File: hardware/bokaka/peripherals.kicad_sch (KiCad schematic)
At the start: 50 parts, among them U1 IS31FL3236A-QFLS2-TR

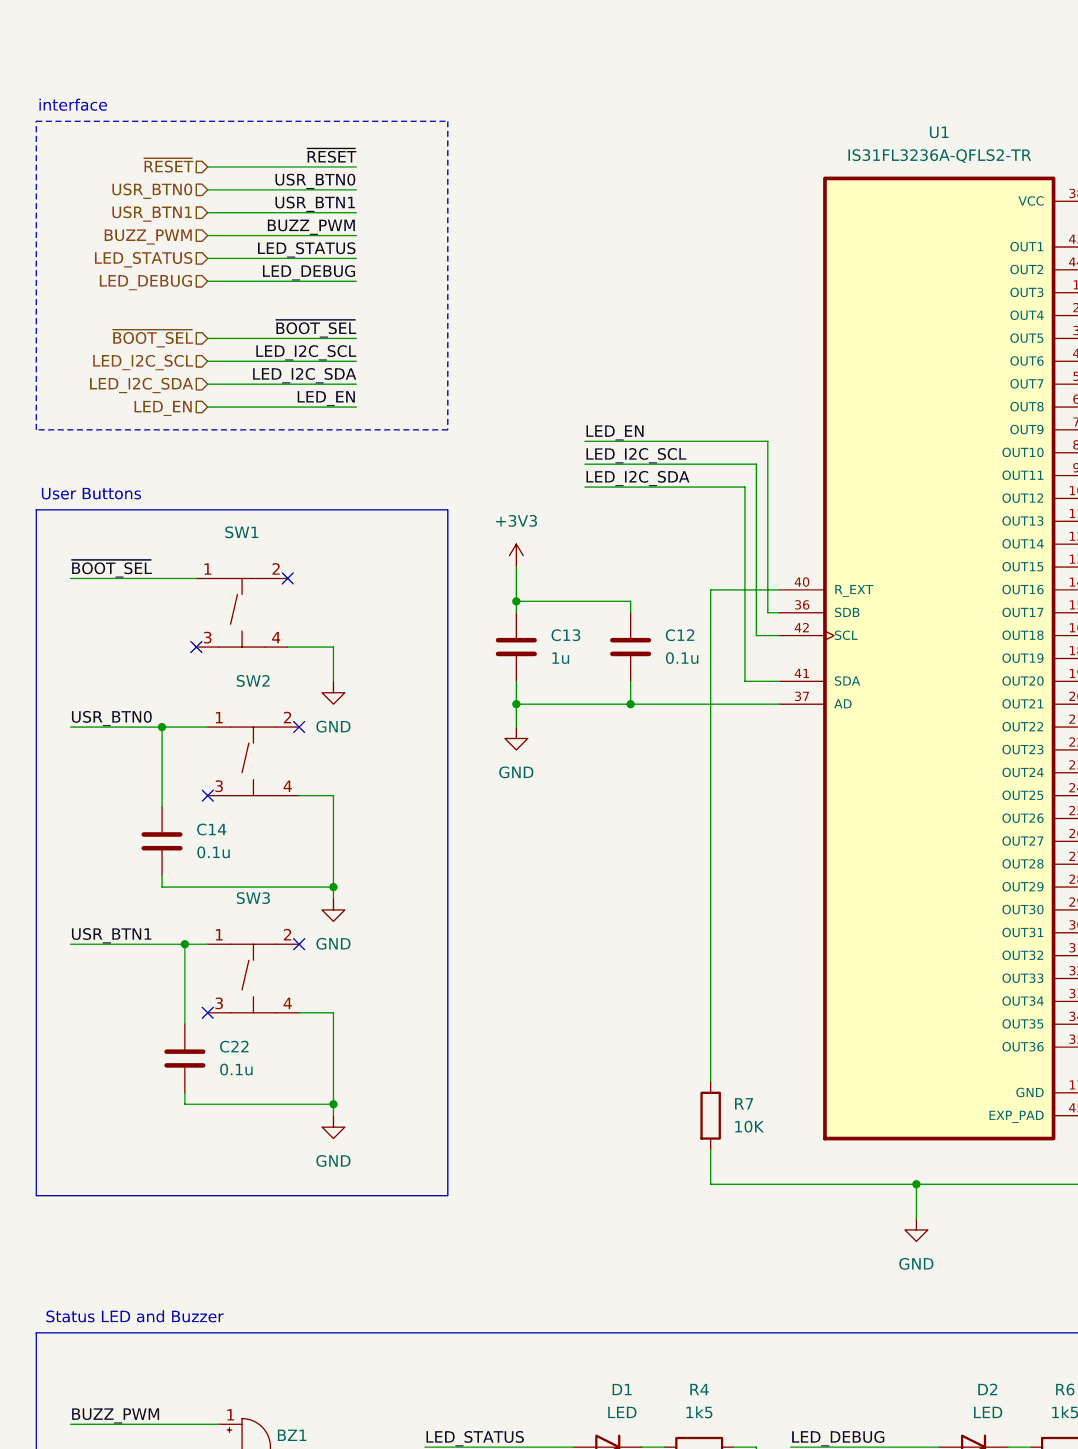
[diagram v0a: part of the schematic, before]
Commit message: hardware update
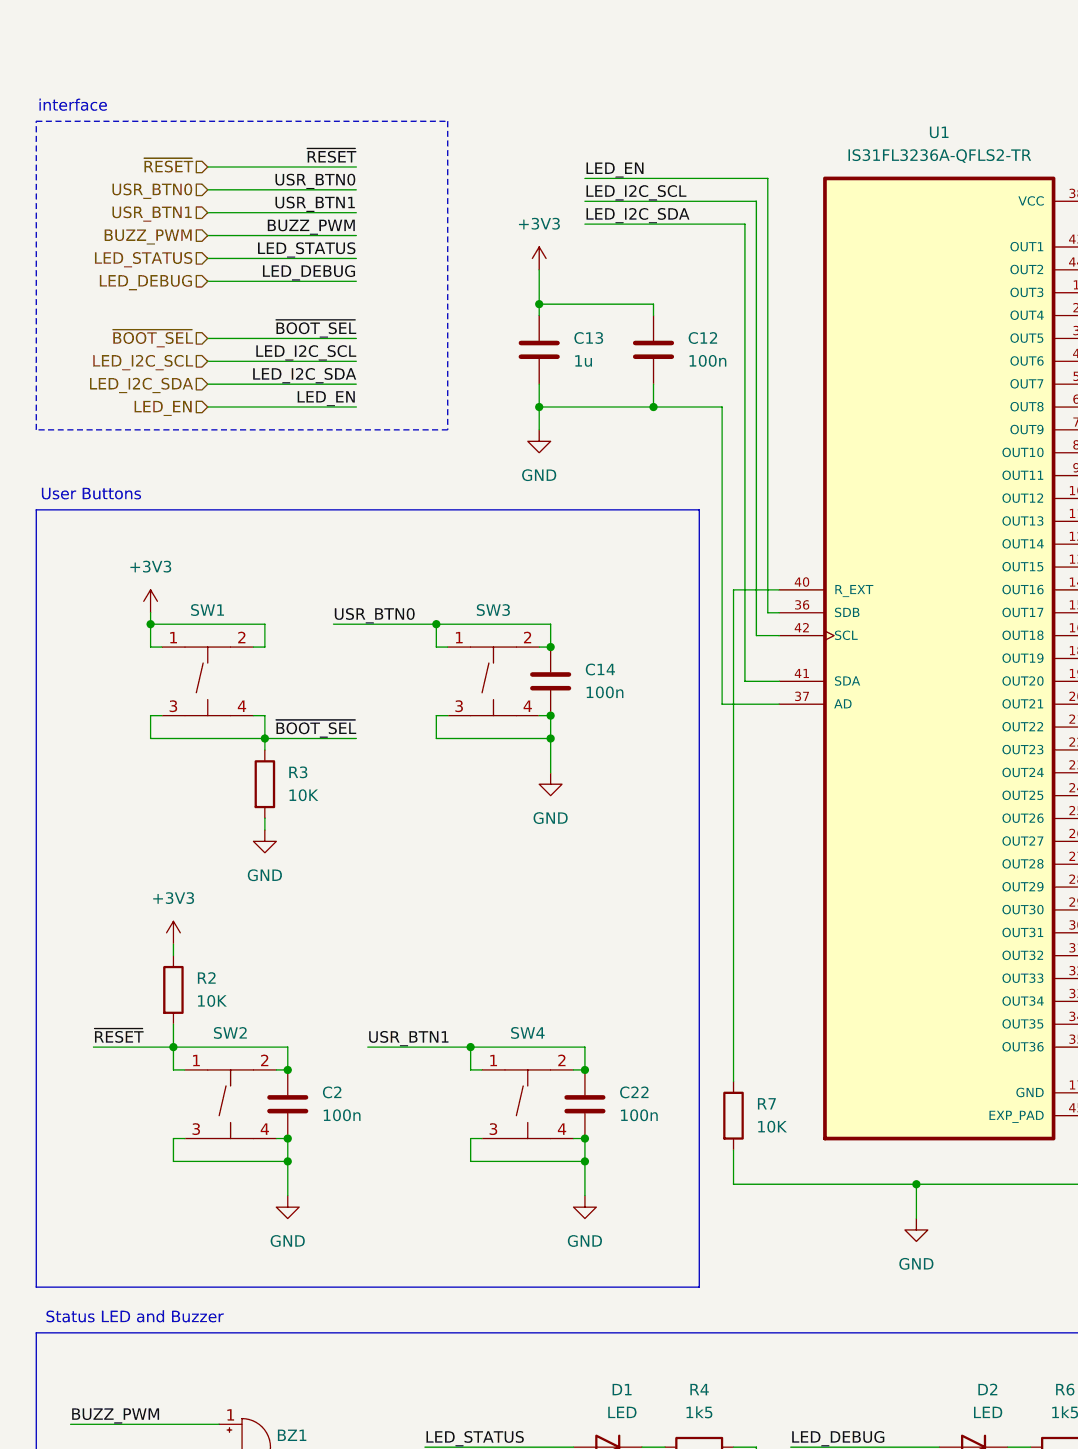
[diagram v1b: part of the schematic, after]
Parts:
- added C2: 100n, Capacitor_SMD:C_0402_1005Metric, symbol Device:C
- added R2, R3: 10K, Resistor_SMD:R_0402_1005Metric, symbol Device:R
- added SW4: ~, EasyEDA_Lib:SW-SMD_4P-L5.1-W5.1-P3.70-LS6.5-TL_H1.5, symbol Symbols:TS-1187A-B-A-B
- C12, C14, C22: value 0.1u -> 100n
- C13: footprint Capacitor_SMD:C_0402_1005Metric -> Capacitor_SMD:C_0603_1608Metric
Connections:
- net +3V3: now also SW1.1 (A), SW1.2 (B), R2.1
- net GND: now also SW2.3 (C), SW3.3 (C), C2.2, R3.2, SW4.3 (C), SW4.4 (D); no longer SW1.4 (D)
- net USR_BTN0: now also SW3.1 (A), SW3.2 (B); no longer SW2.1 (A)
- net USR_BTN1: now also SW4.1 (A), SW4.2 (B); no longer SW3.1 (A)
- net ~{BOOT_SEL}: now also SW1.3 (C), SW1.4 (D), R3.1; no longer SW1.1 (A)
- net ~{RESET}: now also SW2.1 (A), SW2.2 (B), C2.1, R2.2
- no-connect marks 6 -> 0
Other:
- moved on the sheet: C12, C13, R7, SW1

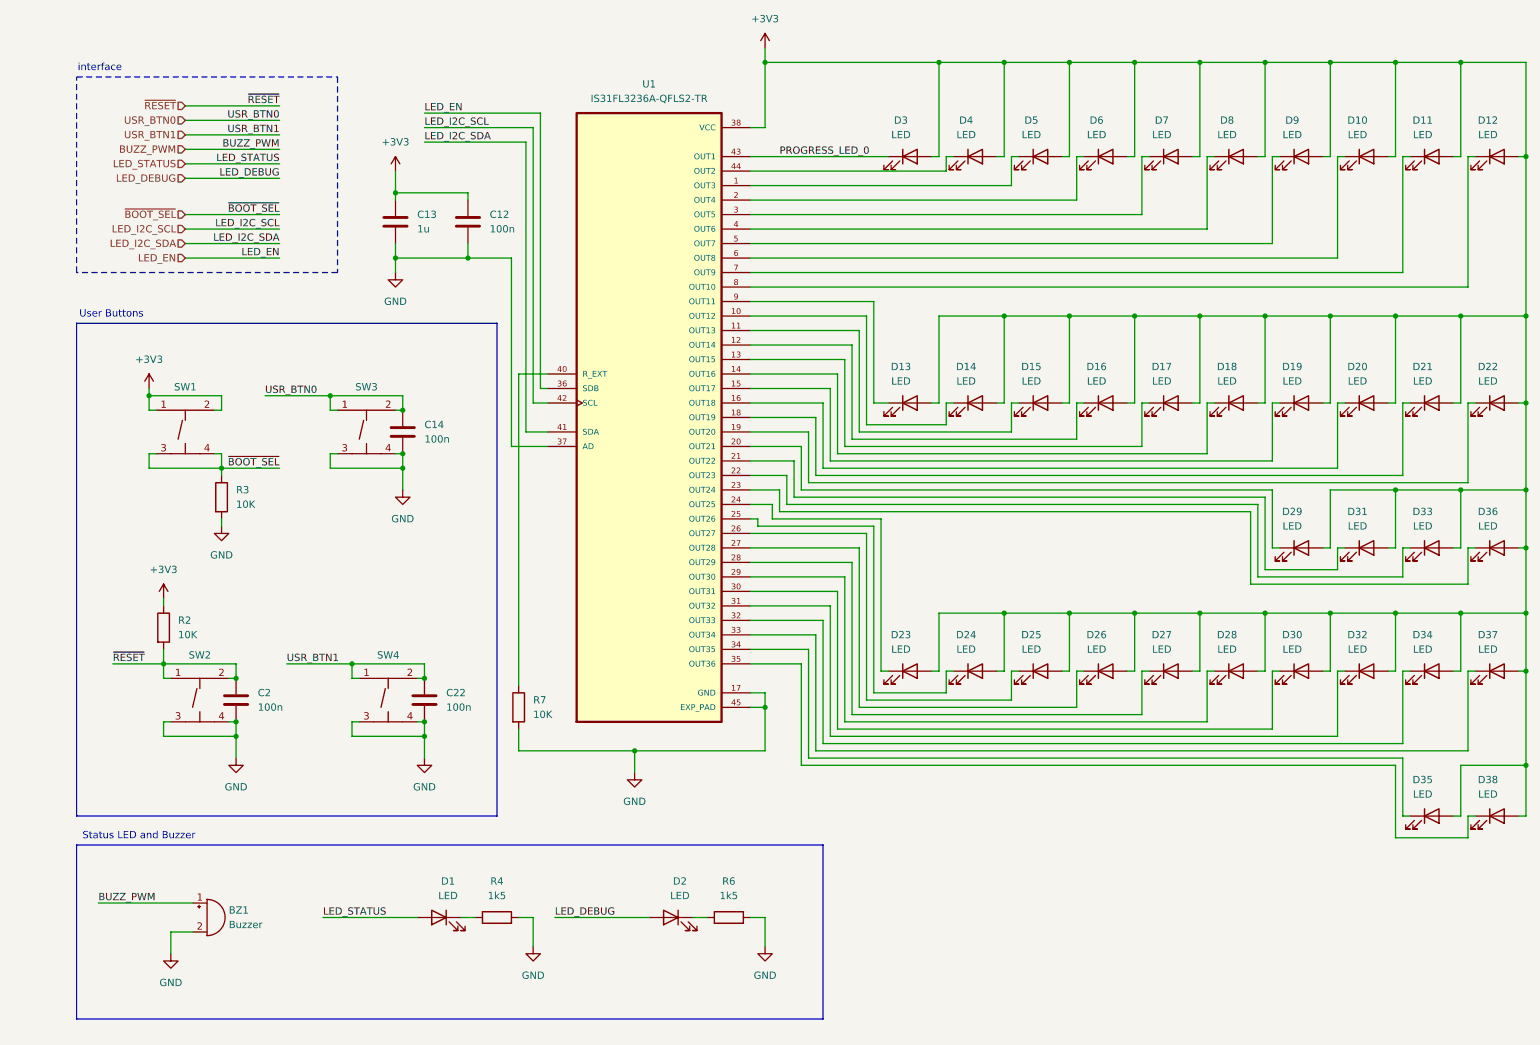
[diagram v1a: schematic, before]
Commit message: Devkit Production Ready
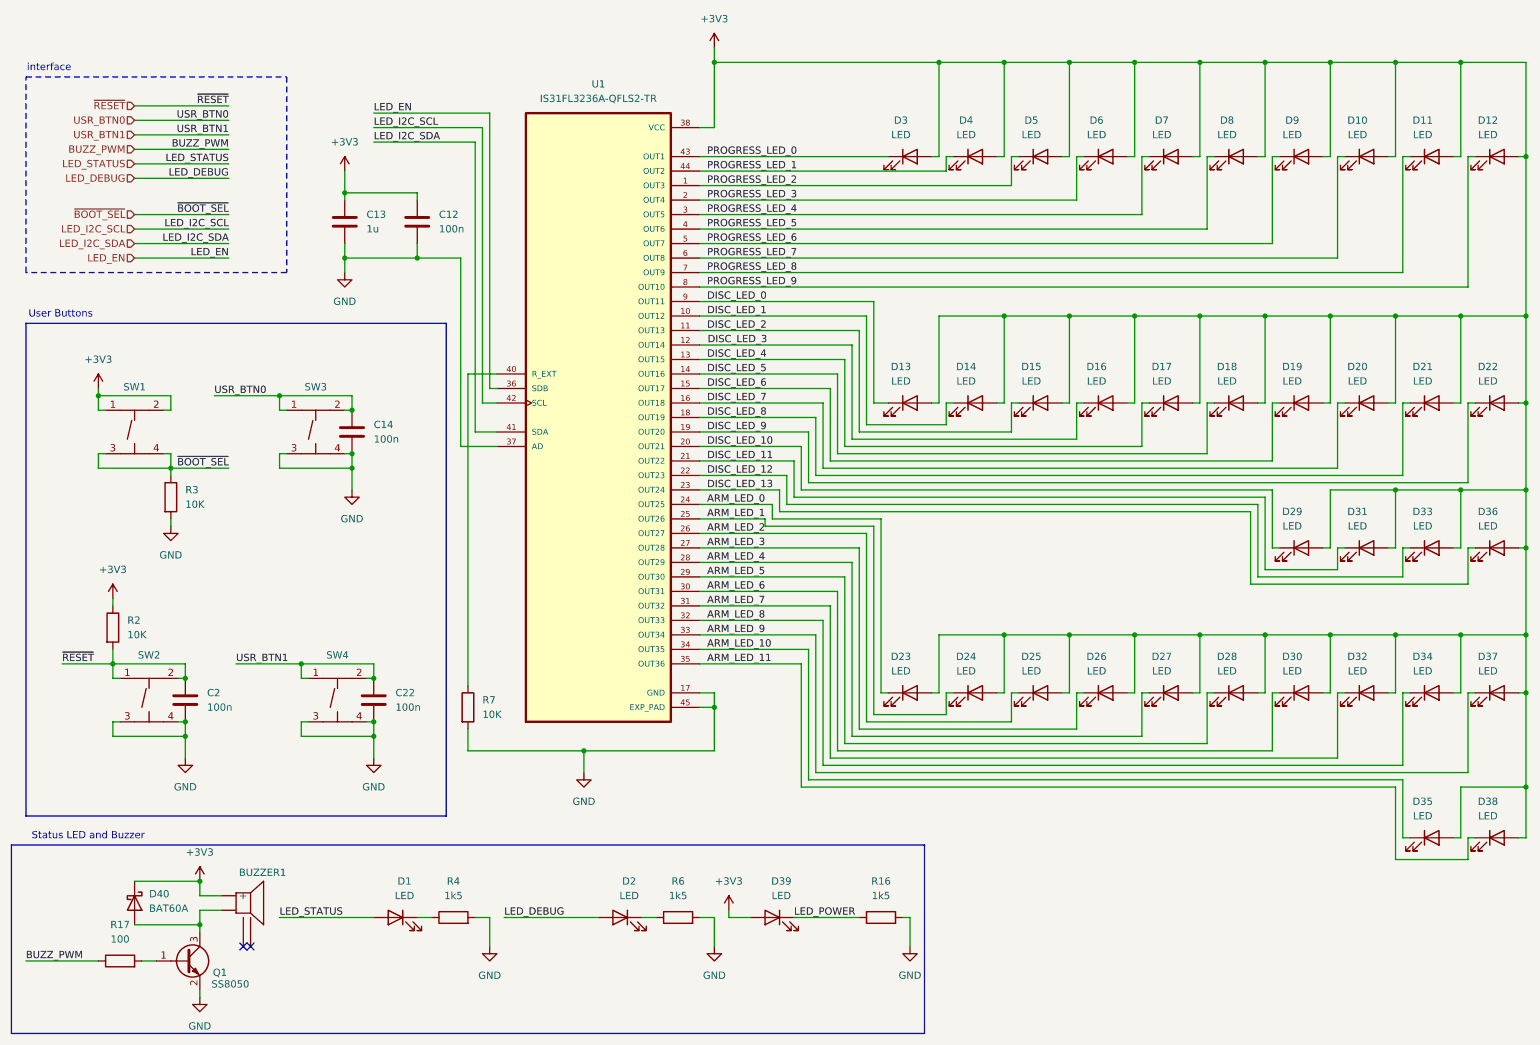
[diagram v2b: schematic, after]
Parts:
- removed BZ1: Buzzer, Footprints:CUI_CPT-9019S-SMT, symbol Device:Buzzer
- added BUZZER1: ~, EasyEDA_Lib:BUZ-SMD_4P-L8.5-W8.5-P8.50-BR, symbol EasyEDA_Lib:MLT-8530
- added D39: LED, LED_SMD:LED_0603_1608Metric, symbol Device:LED
- added D40: BAT60A, Diode_SMD:D_SOD-323, symbol Diode:BAT60A
- added Q1: SS8050, Package_TO_SOT_SMD:SOT-23, symbol Transistor_BJT:SS8050
- added R16: 1k5, Resistor_SMD:R_0402_1005Metric, symbol Device:R
- added R17: 100, Resistor_SMD:R_0402_1005Metric, symbol Device:R
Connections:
- net +3V3: now also BUZZER1.1 (+), D39.2 (A), D40.1 (K)
- net BUZZ_PWM: now also R17.1
- net GND: now also Q1.2 (E), R16.2
- net PROGRESS_LED_2: now reaches D5.1 (K), U1.1 (OUT3)
- net ARM_LED_4: now reaches D27.1 (K), U1.28 (OUT29)
- net DISC_LED_4: now reaches D17.1 (K), U1.13 (OUT15)
- net DISC_LED_5: now reaches D18.1 (K), U1.14 (OUT16)
- net ARM_LED_2: now reaches D25.1 (K), U1.26 (OUT27)
- net DISC_LED_1: now reaches D14.1 (K), U1.10 (OUT12)
- net DISC_LED_2: now reaches D15.1 (K), U1.11 (OUT13)
- net DISC_LED_0: now reaches D13.1 (K), U1.9 (OUT11)
- net DISC_LED_7: now reaches D20.1 (K), U1.16 (OUT18)
- net PROGRESS_LED_8: now reaches D11.1 (K), U1.7 (OUT9)
- net ARM_LED_3: now reaches D26.1 (K), U1.27 (OUT28)
- net PROGRESS_LED_3: now reaches D6.1 (K), U1.2 (OUT4)
- net DISC_LED_3: now reaches D16.1 (K), U1.12 (OUT14)
- net DISC_LED_6: now reaches D19.1 (K), U1.15 (OUT17)
- net ARM_LED_11: now reaches D38.1 (K), U1.35 (OUT36)
- net PROGRESS_LED_4: now reaches D7.1 (K), U1.3 (OUT5)
- net DISC_LED_12: now reaches D33.1 (K), U1.22 (OUT23)
- net ARM_LED_5: now reaches D28.1 (K), U1.29 (OUT30)
- net DISC_LED_9: now reaches D22.1 (K), U1.19 (OUT20)
- net DISC_LED_8: now reaches D21.1 (K), U1.18 (OUT19)
- net ARM_LED_7: now reaches D32.1 (K), U1.31 (OUT32)
- net ARM_LED_0: now reaches D23.1 (K), U1.24 (OUT25)
- net PROGRESS_LED_6: now reaches D9.1 (K), U1.5 (OUT7)
- net PROGRESS_LED_9: now reaches D12.1 (K), U1.8 (OUT10)
- net DISC_LED_10: now reaches D29.1 (K), U1.20 (OUT21)
- net DISC_LED_11: now reaches D31.1 (K), U1.21 (OUT22)
- net DISC_LED_13: now reaches D36.1 (K), U1.23 (OUT24)
- net ARM_LED_1: now reaches D24.1 (K), U1.25 (OUT26)
- net ARM_LED_6: now reaches D30.1 (K), U1.30 (OUT31)
- net ARM_LED_8: now reaches D34.1 (K), U1.32 (OUT33)
- net ARM_LED_9: now reaches D37.1 (K), U1.33 (OUT34)
- net ARM_LED_10: now reaches D35.1 (K), U1.34 (OUT35)
- net PROGRESS_LED_5: now reaches D8.1 (K), U1.4 (OUT6)
- net PROGRESS_LED_1: now reaches D4.1 (K), U1.44 (OUT2)
- net PROGRESS_LED_7: now reaches D10.1 (K), U1.6 (OUT8)
- new net: Q1.1 (B), R17.2
- new net: BUZZER1.2, D40.2 (A), Q1.3 (C)
- new net LED_POWER: D39.1 (K), R16.1
- no-connect marks 0 -> 2
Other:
- moved on the sheet: C12, C13, C14, C2, C22, D1, D2, D23, D24, D25, D26, D27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
